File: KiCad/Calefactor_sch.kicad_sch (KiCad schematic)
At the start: 3 parts, among them U1 SHTC3

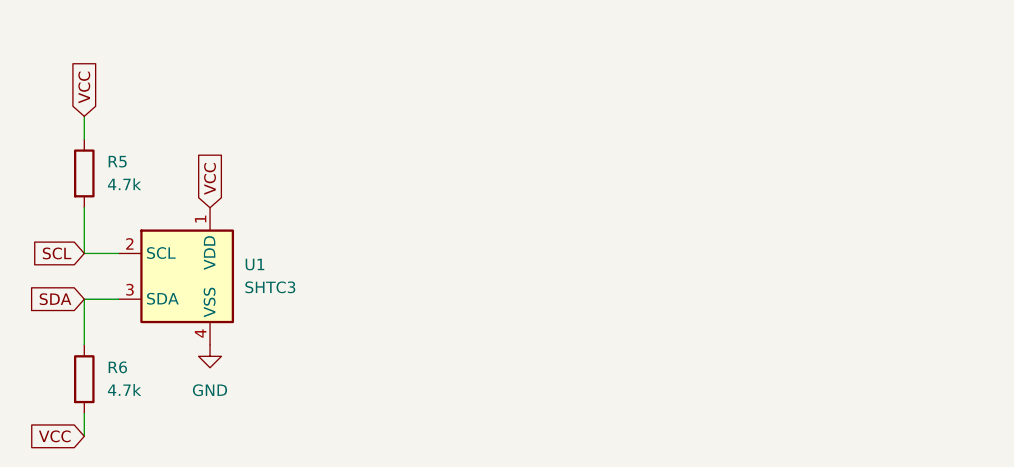
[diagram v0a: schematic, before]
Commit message: calefactor-Usart
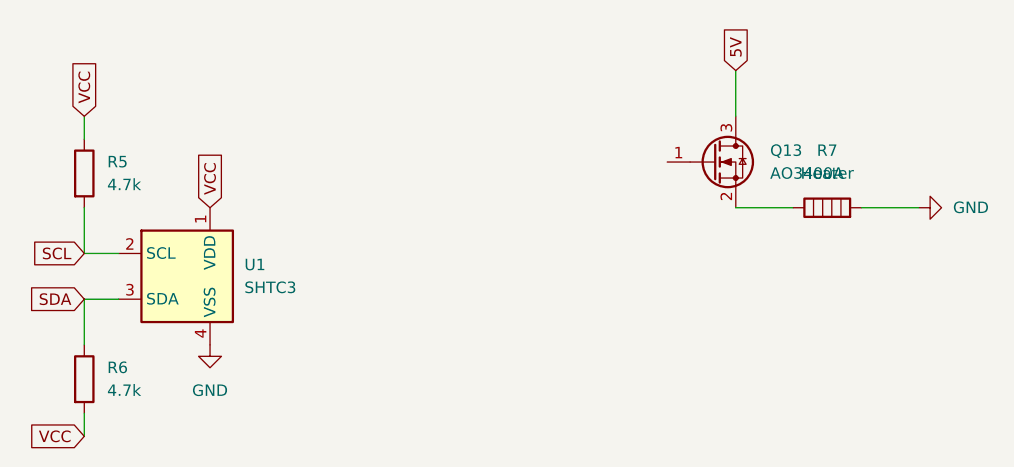
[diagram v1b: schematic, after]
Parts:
- added Q13: AO3400A, Package_TO_SOT_SMD:SOT-23, symbol Transistor_FET:AO3400A
- added R7: Heater, symbol Device:Heater
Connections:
- net GND: now also R7.2
- new net: Q13.2 (S), R7.1
- new net 5V: Q13.3 (D)
